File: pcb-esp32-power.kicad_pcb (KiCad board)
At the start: 2 copper layers, 48.6 x 47.4 mm, 35 parts, among them IC1 IP5108, IC2 SY8008B, J1 C-OBD-II-16M, J2 Conn_01x02, J3 Bus_Connector, U1 STEPDOWN12_5

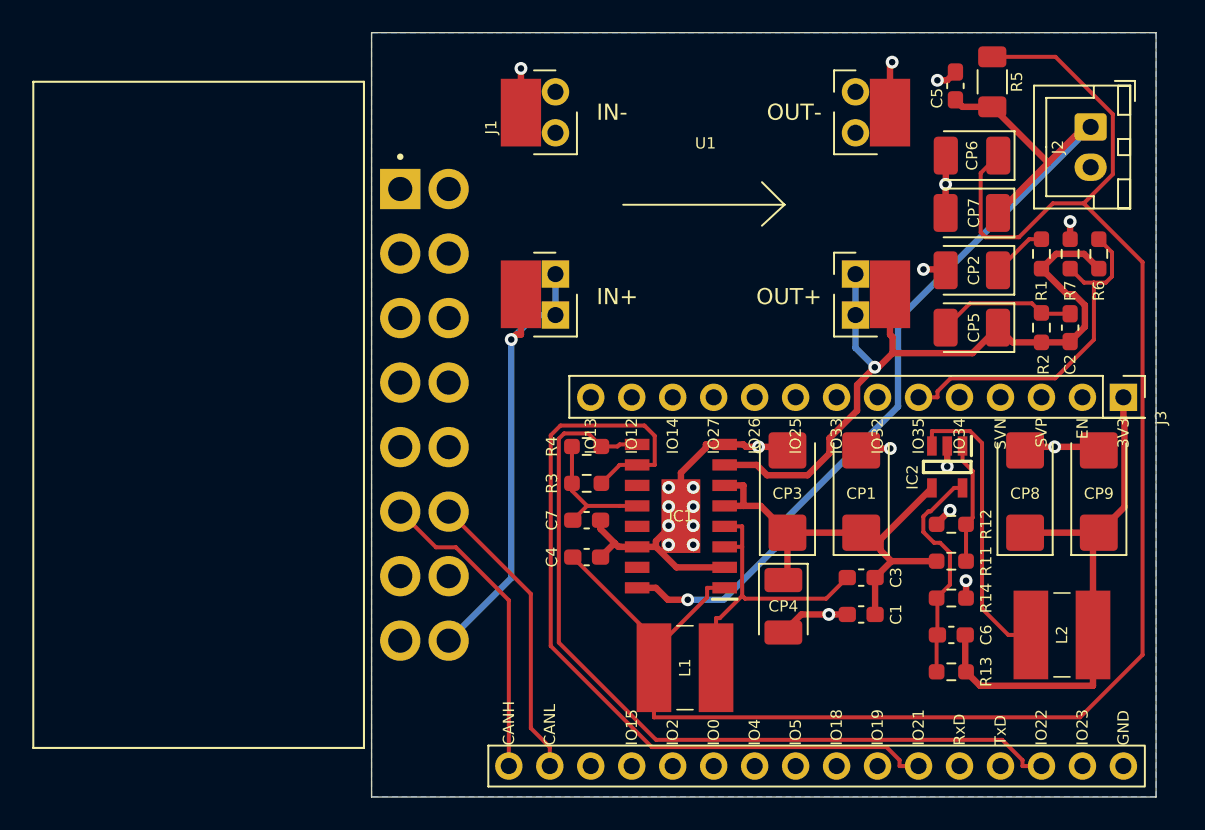
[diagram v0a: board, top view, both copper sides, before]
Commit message: Mit SY8008
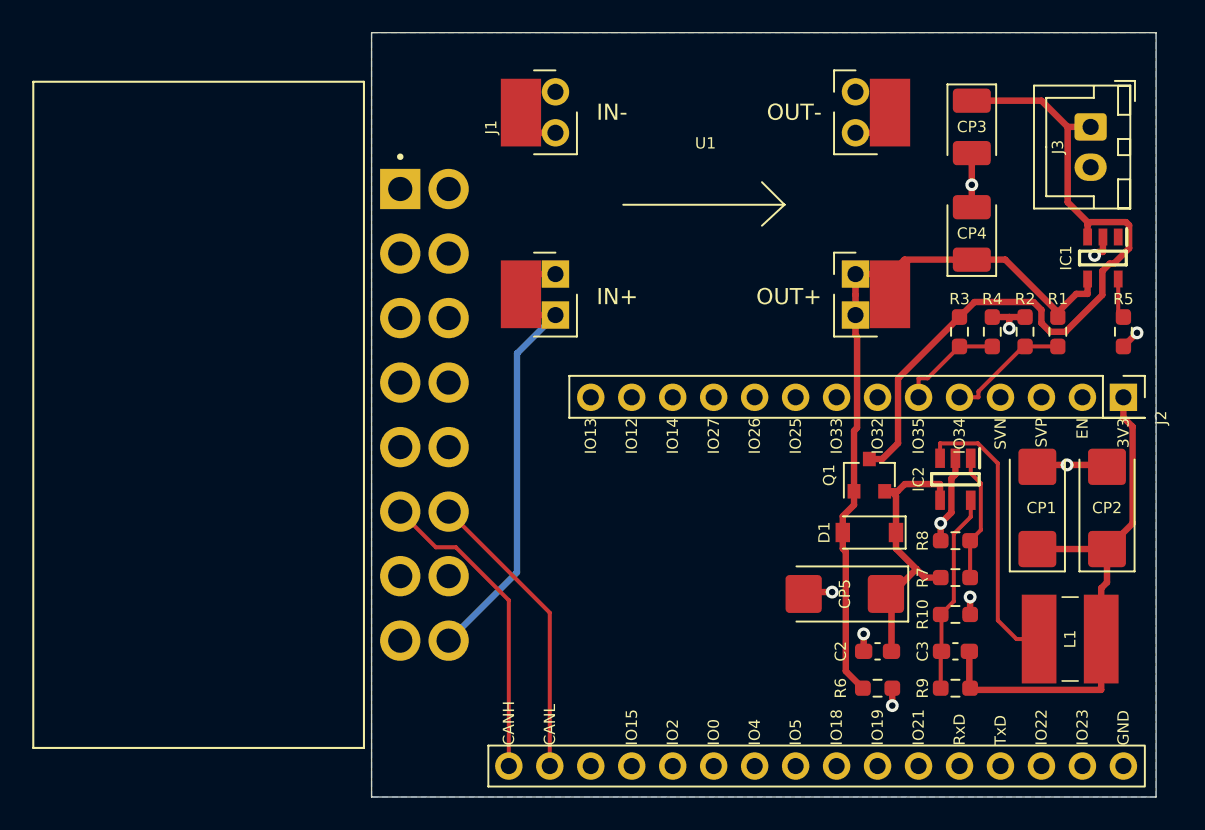
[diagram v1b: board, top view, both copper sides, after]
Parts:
- removed C1, C4, C5: 104, Capacitor_SMD:C_0603_1608Metric_Pad1.08x0.95mm_HandSolder
- removed C6: 47pF, Capacitor_SMD:C_0603_1608Metric_Pad1.08x0.95mm_HandSolder
- removed C7: 2.2uF, Capacitor_SMD:C_0603_1608Metric_Pad1.08x0.95mm_HandSolder
- removed CP6, CP7: 10uF, Capacitor_Tantalum_SMD:CP_EIA-3528-21_Kemet-B_Pad1.50x2.35mm_HandSolder
- removed CP8, CP9: 22uF, Capacitor_Tantalum_SMD:CP_EIA-6032-28_Kemet-C_Pad2.25x2.35mm_HandSolder
- removed L2: 2.2uH, IP5108:CD54_Inductor
- removed the R1 at (167.9, 100.3)
- removed R11, R12: 100k, Resistor_SMD:R_0603_1608Metric_Pad0.98x0.95mm_HandSolder
- removed R13: 453k 1%, Resistor_SMD:R_0603_1608Metric_Pad0.98x0.95mm_HandSolder
- removed R14: 100k 1%, Resistor_SMD:R_0603_1608Metric_Pad0.98x0.95mm_HandSolder
- removed the R2 at (167.9, 104.9)
- added D1: B5819W, Diode_SMD:D_SOD-123, F.Cu at (157.2, 117.6)
- added Q1: Si2307BDS, Package_TO_SOT_SMD:SOT-23, F.Cu at (157.2, 114.0)
- added R10: 100k 1%, Resistor_SMD:R_0603_1608Metric_Pad0.98x0.95mm_HandSolder, F.Cu at (162.6, 122.7)
- added R6: 10K, Resistor_SMD:R_0603_1608Metric_Pad0.98x0.95mm_HandSolder, F.Cu at (157.7, 127.3)
- added R7: 100k, Resistor_SMD:R_0603_1608Metric_Pad0.98x0.95mm_HandSolder, F.Cu at (162.6, 120.4)
- added R8: 100k, Resistor_SMD:R_0603_1608Metric_Pad0.98x0.95mm_HandSolder, F.Cu at (162.6, 118.1)
- added R9: 453k 1%, Resistor_SMD:R_0603_1608Metric_Pad0.98x0.95mm_HandSolder, F.Cu at (162.6, 127.3)
- C2: value 104 -> 100nF
- C3: value 4.7nF -> 47pF
- CP2, CP5: value 10uF -> 22uF; footprint Capacitor_Tantalum_SMD:CP_EIA-3528-21_Kemet-B_Pad1.50x2.35mm_HandSolder -> Capacitor_Tantalum_SMD:CP_EIA-6032-28_Kemet-C_Pad2.25x2.35mm_HandSolder
- CP3: value 22uF -> 10uF; footprint Capacitor_Tantalum_SMD:CP_EIA-6032-28_Kemet-C_Pad2.25x2.35mm_HandSolder -> Capacitor_Tantalum_SMD:CP_EIA-3528-21_Kemet-B_Pad1.50x2.35mm_HandSolder
- IC1: value IP5108 -> TP4054-42-SOT25-R; footprint IP5108:IP5108 -> tp4054:SOT95P280X100-5N
- L1: value 1uH -> 2.2uH
- R1: renamed from R6; value R -> 200k
- R2: renamed from R7; value R -> 390k
- R3, R4: value 3.3k -> 470k
- R5: value 10mOhm -> 2K; footprint Resistor_SMD:R_1206_3216Metric_Pad1.30x1.75mm_HandSolder -> Resistor_SMD:R_0603_1608Metric_Pad0.98x0.95mm_HandSolder
- moved IC1 30.7 mm to (171.7, 100.6), turned to 270 degrees
- moved R4 26.1 mm to (164.8, 105.2), turned to 90 degrees
- moved CP4 25.9 mm to (163.6, 99.1), turned to 90 degrees
- moved CP3 25.3 mm to (163.6, 92.5), turned to 270 degrees
- moved R3 25.0 mm to (162.8, 105.2), turned to 270 degrees
- moved L1 23.9 mm to (169.7, 124.2), turned to 270 degrees
- moved C2 23.3 mm to (157.7, 125.0), turned to 180 degrees
- moved CP5 18.3 mm to (155.7, 121.4)
- moved R5 17.5 mm to (173.0, 105.2), turned to 270 degrees
- moved CP2 16.9 mm to (172.0, 116.1), turned to 90 degrees
- moved CP1 11.0 mm to (167.6, 116.1)
- moved C3 7.42 mm to (162.6, 125.0)
- moved R2 5.58 mm to (166.9, 105.2)
- moved R1 5.45 mm to (168.9, 105.2), turned to 270 degrees
- moved IC2 0.92 mm to (162.6, 114.3)
- renumbered J3 to J2, J2 to J3
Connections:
- C2 pad 1: 5VIN -> 5VOUT
- C2 pad 2: Net-(C2-Pad2) -> GND
- C3 pad 1: 5VOUT -> +3V3
- CP1 pad 1: 5VOUT -> +3V3
- CP2 pad 1: Net-(CP2-Pad1) -> +3V3
- CP3 pad 1: 5VOUT -> +BATT
- CP4 pad 1: 5VOUT -> 5VIN
- CP5 pad 1: 5VIN -> 5VOUT
- CP5 pad 2: Net-(C2-Pad2) -> GND
- IC1 pad 1: Net-(C4-Pad1) -> Net-(IC1-Pad1)
- IC1 pad 3: Net-(C3-Pad2) -> +BATT
- IC1 pad 4: Net-(C3-Pad2) -> 5VIN
- IC1 pad 5: 5VOUT -> Net-(IC1-Pad5)
- IC2 pad 5: Net-(C6-Pad2) -> Net-(C3-Pad2)
- J2 pad 5: Net-(J3-Pad5) -> EXTPOW
- J2 pad 6: EXTPOW -> BATTVOLT
- L1 pad 1: Net-(C4-Pad1) -> +3V3
- L1 pad 2: Net-(C3-Pad2) -> Net-(IC2-Pad3)
- R3 pad 1: Net-(C7-Pad1) -> +BATT
- R3 pad 2: SDA -> BATTVOLT
- R4 pad 1: Net-(C7-Pad1) -> BATTVOLT
- R4 pad 2: SCL -> GND
- R5 pad 1: +BATT -> Net-(IC1-Pad5)
- R5 pad 2: Net-(C4-Pad1) -> GND
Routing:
- net Net-(C4-Pad1): track 107.3 -> 0.00 mm
- net SDA: track 51.7 -> 0.00 mm
- net SCL: track 51.3 -> 0.00 mm
- net GND: track 51.2 -> 29.5 mm, vias 21 -> 10
- net EXTPOW: track 21.9 -> 7.62 mm
- net Net-(C6-Pad2): track 14.1 -> 0.00 mm
- net +BATT: track 59.7 -> 46.3 mm, vias 1 -> 0
- net 5VOUT: track 28.7 -> 17.9 mm
- net Net-(C2-Pad2): track 8.61 -> 0.00 mm
- net Net-(C7-Pad1): track 8.43 -> 0.00 mm
- net BATTVOLT: track 0.00 -> 6.57 mm
- net Net-(C3-Pad2): track 18.9 -> 12.5 mm
- net Net-(CP2-Pad1): track 3.49 -> 0.00 mm
- net Net-(IC1-Pad5): track 0.00 -> 2.49 mm
- net 5VIN: track 47.9 -> 45.6 mm, vias 1 -> 0
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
